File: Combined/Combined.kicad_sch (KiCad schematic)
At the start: 13 parts, among them U1 ATMEGA168PA-MU, U2 RA-08H(915), U3 ATGM336H-5N31, U4 X1B000301000200

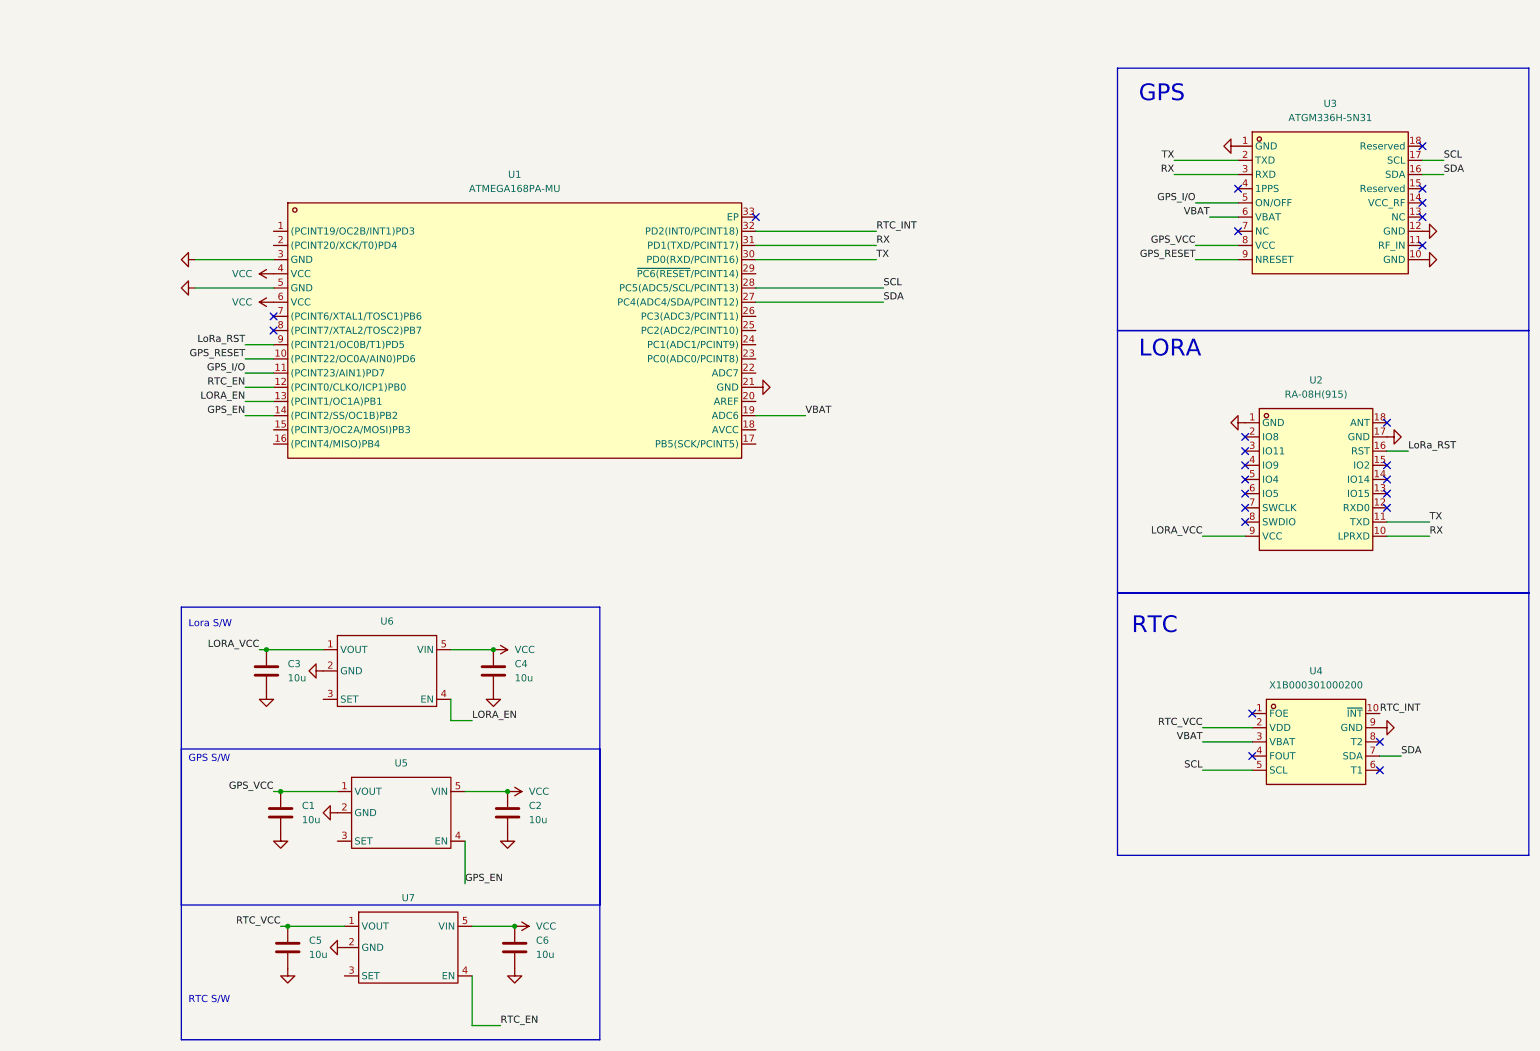
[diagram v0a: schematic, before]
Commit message: Working.
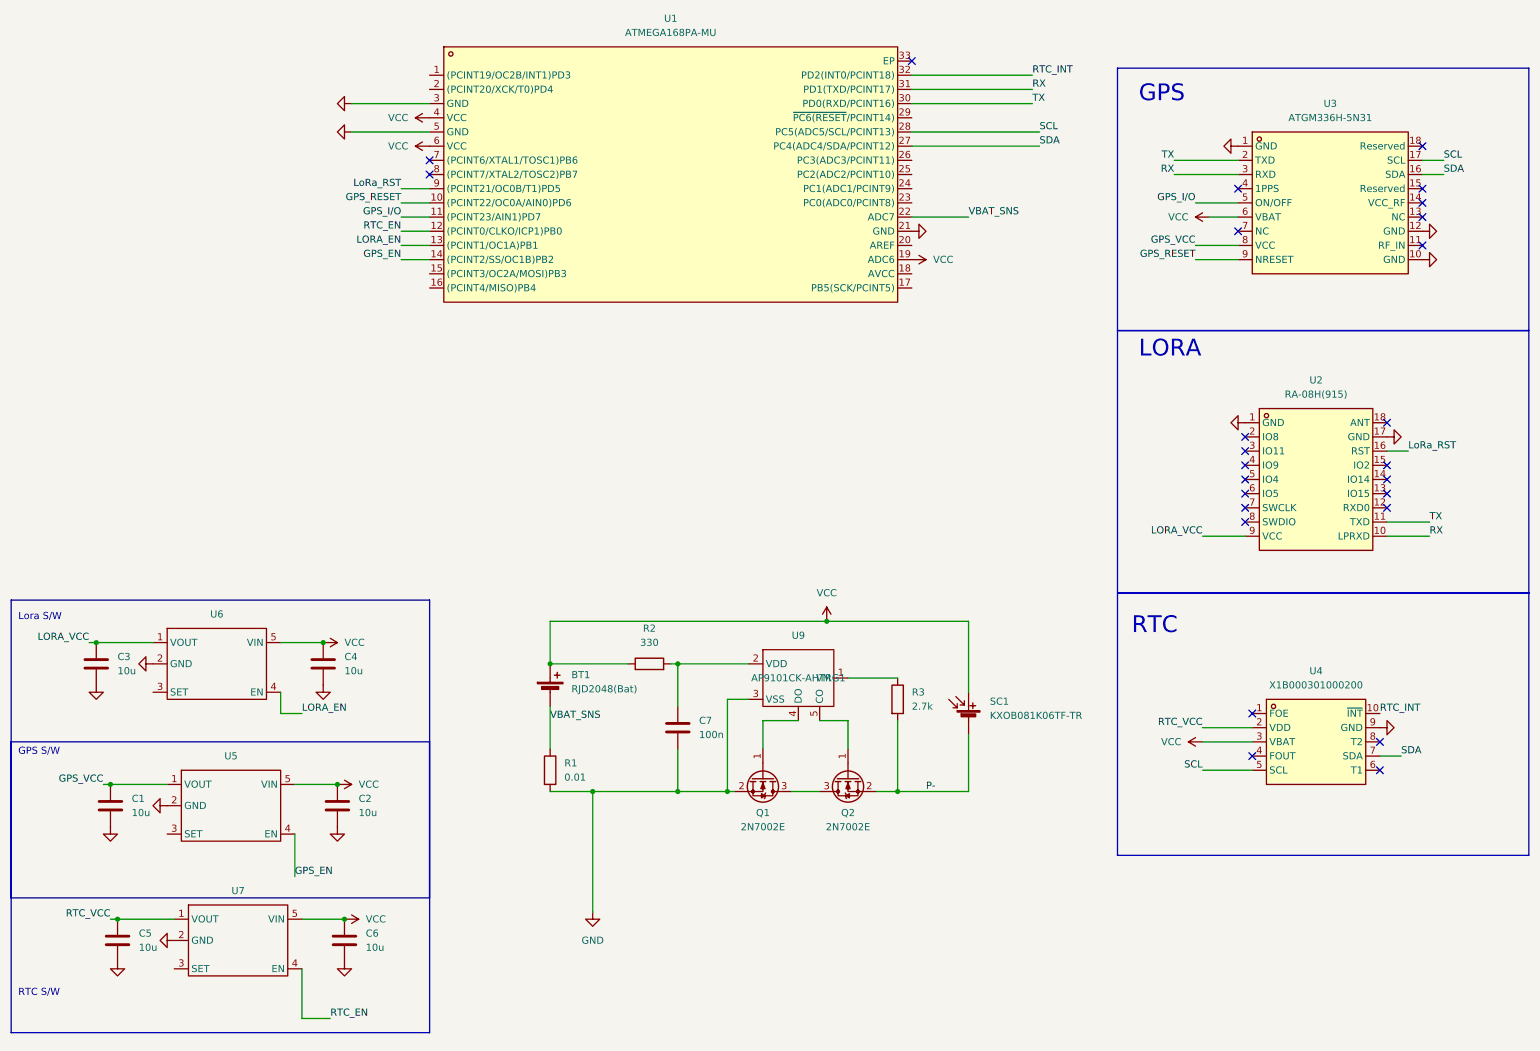
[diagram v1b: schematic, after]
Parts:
- added BT1: RJD2048(Bat), Connector_PinHeader_2.54mm:PinHeader_1x02_P2.54mm_Vertical, symbol Device:Battery_Cell
- added C7: 100n, symbol Device:C
- added Q1, Q2: 2N7002E, Package_TO_SOT_SMD:SOT-23, symbol Transistor_FET:2N7002E
- added R1: 0.01, Resistor_SMD:R_0805_2012Metric, symbol Device:R
- added R2: 330, symbol Device:R
- added R3: 2.7k, symbol Device:R
- added SC1: KXOB081K06TF-TR, Connector_PinHeader_2.54mm:PinHeader_1x02_P2.54mm_Vertical, symbol Device:Solar_Cell
- added U9: AP9101CK-AHTRG1, PARTS:SOT-23-5_L3.0-W1.7-P0.95-LS2.8-BL, symbol PARTS:AP9101C
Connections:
- net VBAT is gone; now on net VCC: U1.19 (ADC6), U3.6 (VBAT), U4.3 (VBAT)
- net GND: now also C7.2, Q1.2 (S), R1.2, U9.3 (VSS)
- net VCC: now also BT1.1 (+), R2.1, SC1.1 (+)
- net VBAT_SNS: now reaches U1.22 (ADC7)
- net VBAT_SNS: now also BT1.2 (-), R1.1
- new net: C7.1, R2.2, U9.2 (VDD)
- new net: Q2.1 (G), U9.5 (CO)
- new net: Q1.3 (D), Q2.3 (D)
- new net: Q1.1 (G), U9.4 (DO)
- new net: R3.1, U9.1 (VM)
- new net P-: Q2.2 (S), R3.2, SC1.2 (-)
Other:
- moved on the sheet: C1, C2, C3, C4, C5, C6, U1, U5, U6, U7
